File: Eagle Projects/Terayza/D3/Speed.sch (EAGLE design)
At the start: 36 parts, among them Q2 16MHz, Q3 16MHz, U1 ATMEGA328P-AU, U2 MCP2551, X1 5566-6, X2 5566-6

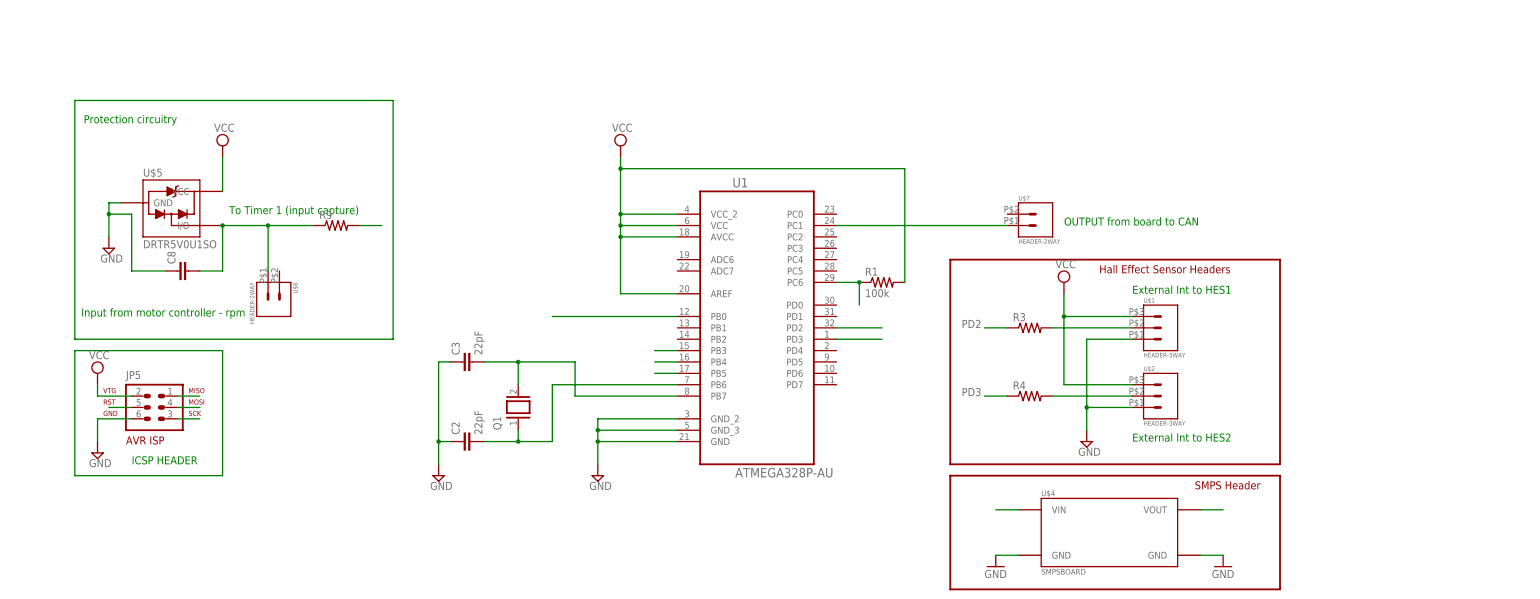
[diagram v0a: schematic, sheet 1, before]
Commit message: Helped with T board
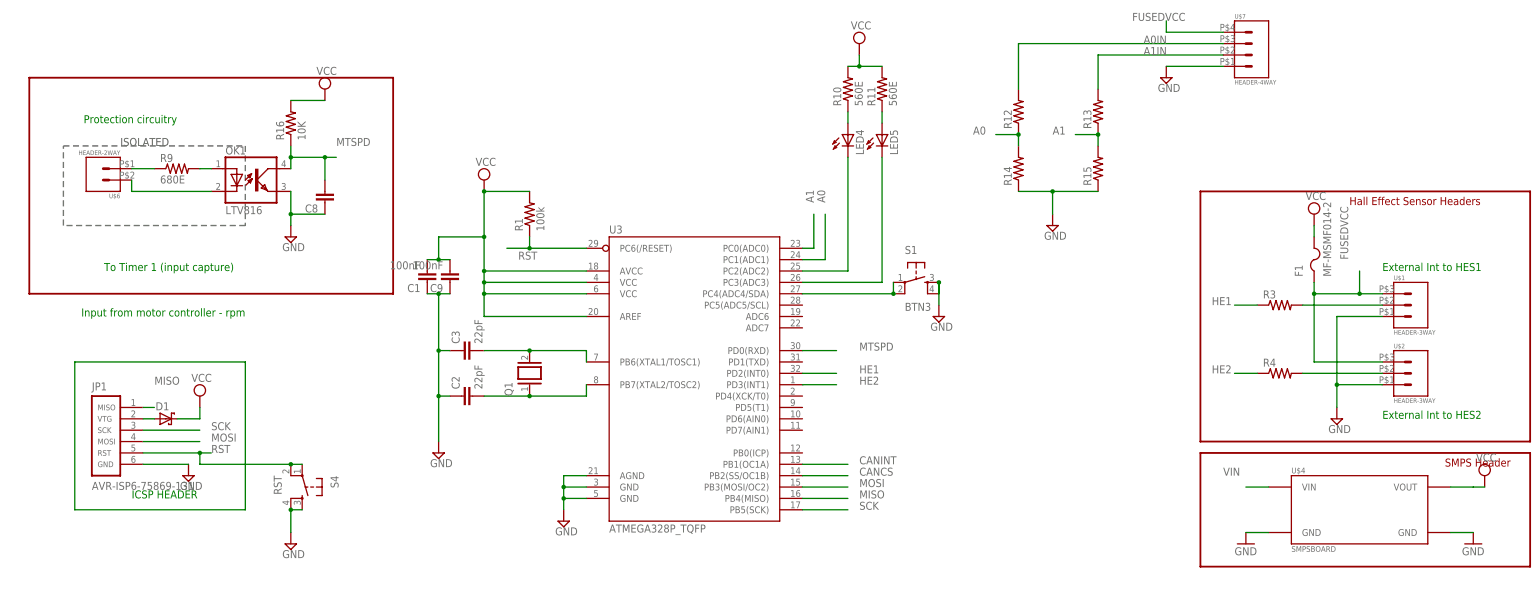
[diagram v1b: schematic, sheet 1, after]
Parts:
- removed JP5: AVR-ISP-6, avr-6:AVR-ISP-6
- removed U$5: DRTR5V0U1SO, RobThePyro:DRTR5V0U1SO
- removed U1: ATMEGA328P-AU, Atmel_By_element14_Batch_1-00:ATMEGA328P-AU
- added C1, C9: 100nF, resistor:C-EUC0805
- added D1: (no value), diode:SCHOTTKY-DIODESMD
- added F1: MF-MSMF014-2, adafruit:PTCFUSE-1812
- added JP1: AVR-ISP6-75869-131, atmel-avr:AVR-ISP6-75869-131
- added LED4, LED5: (no value), led:LEDCHIP-LED0805
- added OK1: LTV816, optocoupler:LTV816
- added R10, R11: 560E, resistor:R-US_M0805
- added R12, R13, R14, R15: (no value), resistor:R-US_M0805
- added R16: 10K, resistor:R-US_M0805
- added S1: BTN3, SparkFun:TAC_SWITCHSMD
- added S4: RST, SparkFun:TAC_SWITCHSMD
- added U3: ATMEGA328P_TQFP, SparkFun-DigitalIC:ATMEGA328P_TQFP
- R9: value (none) -> 680E
- U$7: value HEADER-2WAY -> HEADER-4WAY; device con-TE-EP:HEADER-2WAY -> con-TE-EP:HEADER-4WAY
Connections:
- removed net PB0: R9.2, U1.PB0
- new net A0: R12.1, R14.2, U3.PC1(ADC1)
- new net A0IN: R12.2, U$7.P$3
- new net A1: R13.1, R15.2, U3.PC0(ADC0)
- new net A1IN: R13.2, U$7.P$2
- new net FUSEDVCC: F1.1, U$1.P$3, U$2.P$3, U$7.P$4
- new net HE1: R3.1, U3.PD2(INT0)
- new net HE2: R4.1, U3.PD3(INT1)
- new net MTSPD: C8.2, OK1.COL, R16.1, U3.PD0(RXD)
- new net N$10: LED5.C, U3.PC3(ADC3)
- new net N$2: D1.A, JP1.2
- new net N$5: C3.2, Q1.2, U3.PB6(XTAL1/TOSC1)
- new net N$6: C2.2, Q1.1, U3.PB7(XTAL2/TOSC2)
- new net N$9: LED4.C, U3.PC2(ADC2)
- net CANCS: now also U3.PB2(SS/OC1B)
- net CANINT: now also U3.PB1(OC1A)
- net GND: now also C1.1, C9.1, JP1.6, OK1.EMIT, R14.1, R15.1, S1.3, S1.4, S4.3, S4.4, U$7.P$1, U3.AGND, U3.GND@3, U3.GND@5; no longer JP5.6, U$5.GND, U1.GND, U1.GND_2, U1.GND_3
- net MISO: now also JP1.1, U3.PB4(MISO); no longer JP5.1, U1.PB4
- net MOSI: now also JP1.4, U3.PB3(MOSI/OC2); no longer JP5.4, U1.PB3
- net N$11: now also S1.1, S1.2, U3.PC4(ADC4/SDA); no longer U$4.VIN
- net N$12: now also OK1.C, U$6.P$2; no longer U$4.VOUT
- net N$3: no longer C8.2, U$5.I/O
- net N$4: now also OK1.A, R9.2; no longer U$7.P$1, U1.PC1
- net N$7: now also LED4.A, R10.1; no longer C3.2, Q1.2, U1.PB7
- net N$8: now also LED5.A, R11.1; no longer C2.2, Q1.1, U1.PB6
- net PD2: no longer R3.1, U1.PD2
- net PD3: no longer R4.1, U1.PD3
- net RST: now also JP1.5, S4.1, S4.2, U3.PC6(/RESET); no longer JP5.5, U1.PC6
- net SCK: now also JP1.3, U3.PB5(SCK); no longer JP5.3, U1.PB5
- net VCC: now also C1.2, C9.2, D1.C, F1.2, R10.2, R11.2, R16.2, U$4.VOUT, U3.AREF, U3.AVCC, U3.VCC@4, U3.VCC@6; no longer JP5.2, U$1.P$3, U$2.P$3, U$5.VCC, U1.AREF, U1.AVCC, U1.VCC, U1.VCC_2
- net VIN: now also U$4.VIN
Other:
- note added: "ISOLATED"
- note removed: "OUTPUT from board to CAN"
- moved on the sheet: C2, C3, C8, Q1, R1, R3, R4, R9, U$1, U$2, U$4, U$6
